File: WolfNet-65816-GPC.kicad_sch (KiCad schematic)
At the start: 37 parts, among them J1 Conn_01x01, J2 Conn_01x01, J3 Conn_01x01, J4 Conn_01x01, J5 USB_B, J6 ATX-24, SW1 SW_SPST, SW2 SW_Push, U1 WD65C816S, U10 LM7905_TO220, U11 SC28L91, U12 DS1813, U2 MCP2200-I-SO, U3 74HCT573, U4 74HCT245, U5 AS6C1608, U6 XCR3064XL-VQ100, U7 SST39SF040, U8 SST39SF040, U9 XCR3064XL-VQ100, X1 ACO-12MHz, X2 ACO-3.6864MHz

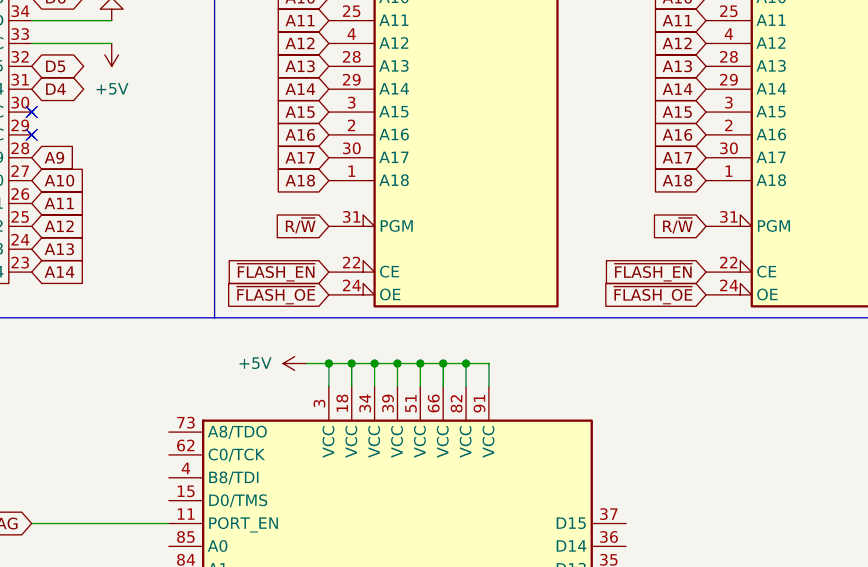
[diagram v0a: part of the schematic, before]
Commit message: Update WolfNet-65816-GPC.kicad_sch
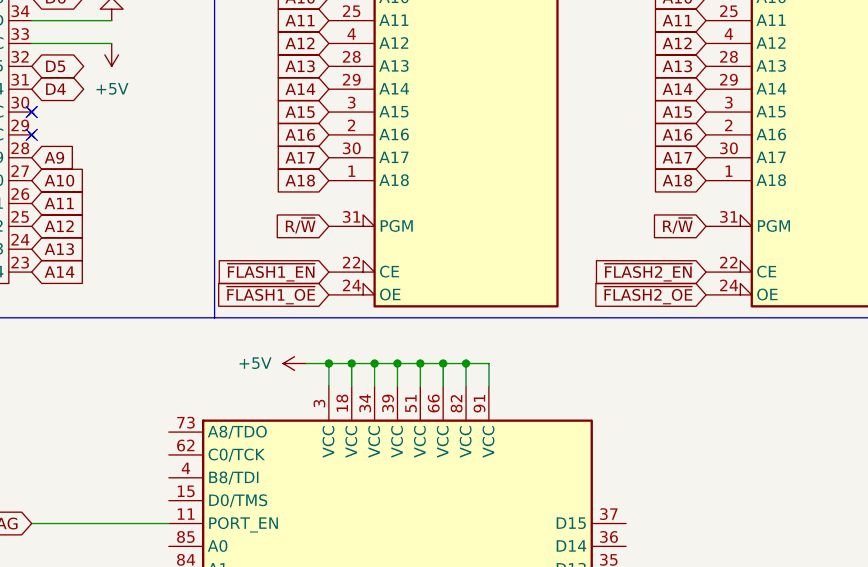
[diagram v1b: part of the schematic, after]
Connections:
- net ~{FLASH_EN} renamed ~{FLASH1_EN}
- net ~{FLASH1_EN}: no longer U8.22 (CE)
- net ~{FLASH_OE} renamed ~{FLASH1_OE}
- net ~{FLASH1_OE}: no longer U8.24 (OE)
- new net ~{FLASH2_EN}: U8.22 (CE)
- new net ~{FLASH2_OE}: U8.24 (OE)
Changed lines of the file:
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@@
     )
   )
-  (global_label "~{FLASH_EN}" (shape input) (at 218.44 78.74 180) (fields_autoplaced)
-    (effects (font (size 1.27 1.27)) (justify right))
-    (property "Intersheet References" "${INTERSHEET_REFS}" (id 0) (at 206.8345 78.6606 0)
+  (global_label "~{FLASH2_EN}" (shape input) (at 218.44 78.74 180) (fields_autoplaced)
+    (effects (font (size 1.27 1.27)) (justify right))
+    (property "Intersheet References" "${INTERSHEET_REFS}" (id 0) (at 205.625 78.6606 0)
       (effects (font (size 1.27 1.27)) (justify right) hide)
     )
@@
     )
   )
-  (global_label "~{FLASH_EN}" (shape input) (at 176.53 78.74 180) (fields_autoplaced)
-    (effects (font (size 1.27 1.27)) (justify right))
-    (property "Intersheet References" "${INTERSHEET_REFS}" (id 0) (at 164.9245 78.6606 0)
+  (global_label "~{FLASH1_EN}" (shape input) (at 176.53 78.74 180) (fields_autoplaced)
+    (effects (font (size 1.27 1.27)) (justify right))
+    (property "Intersheet References" "${INTERSHEET_REFS}" (id 0) (at 163.715 78.6606 0)
       (effects (font (size 1.27 1.27)) (justify right) hide)
     )
@@
     )
   )
-  (global_label "~{FLASH_OE}" (shape input) (at 176.53 81.28 180) (fields_autoplaced)
-    (effects (font (size 1.27 1.27)) (justify right))
-    (property "Intersheet References" "${INTERSHEET_REFS}" (id 0) (at 164.9245 81.2006 0)
+  (global_label "~{FLASH1_OE}" (shape input) (at 176.53 81.28 180) (fields_autoplaced)
+    (effects (font (size 1.27 1.27)) (justify right))
+    (property "Intersheet References" "${INTERSHEET_REFS}" (id 0) (at 163.715 81.2006 0)
       (effects (font (size 1.27 1.27)) (justify right) hide)
     )
@@
     )
   )
-  (global_label "~{FLASH_OE}" (shape input) (at 218.44 81.28 180) (fields_autoplaced)
-    (effects (font (size 1.27 1.27)) (justify right))
-    (property "Intersheet References" "${INTERSHEET_REFS}" (id 0) (at 206.8345 81.2006 0)
-      (effects (font (size 1.27 1.27)) (justify right) hide)
-    )
+  (global_label "~{FLASH2_OE}" (shape input) (at 218.44 81.28 180) (fields_autoplaced)
+    (effects (font (size 1.27 1.27)) (justify right))
+    (property "Intersheet References" "${INTERSHEET_REFS}" (id 0) (at 205.625 81.2006 0)
+      (effects (font (size 1.27 1.27)) (justify right) hide)
+    )
